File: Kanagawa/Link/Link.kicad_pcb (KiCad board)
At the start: 2 copper layers, 23 x 24 mm, 2 parts, among them J0 Conn_02x10_Counter_Clockwise, J1 Conn_02x10_Counter_Clockwise

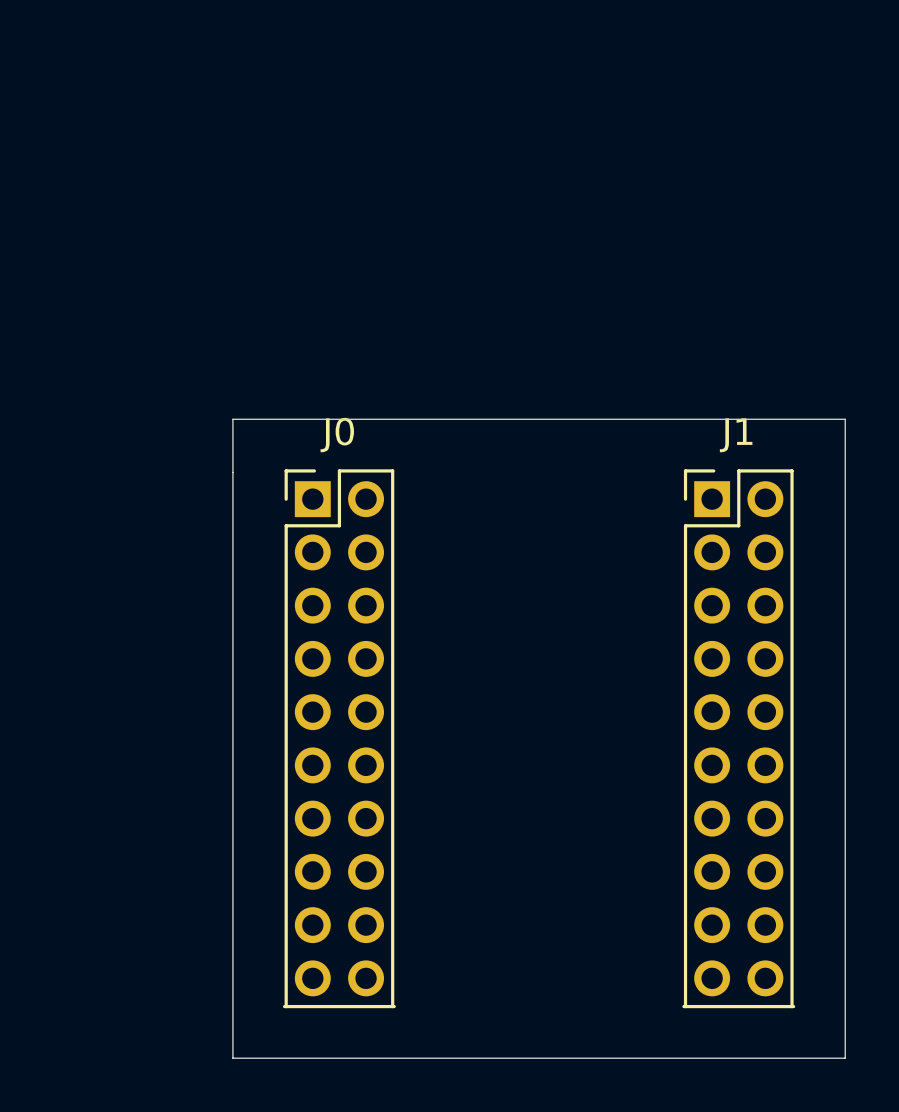
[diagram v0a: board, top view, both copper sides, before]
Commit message: link bridge
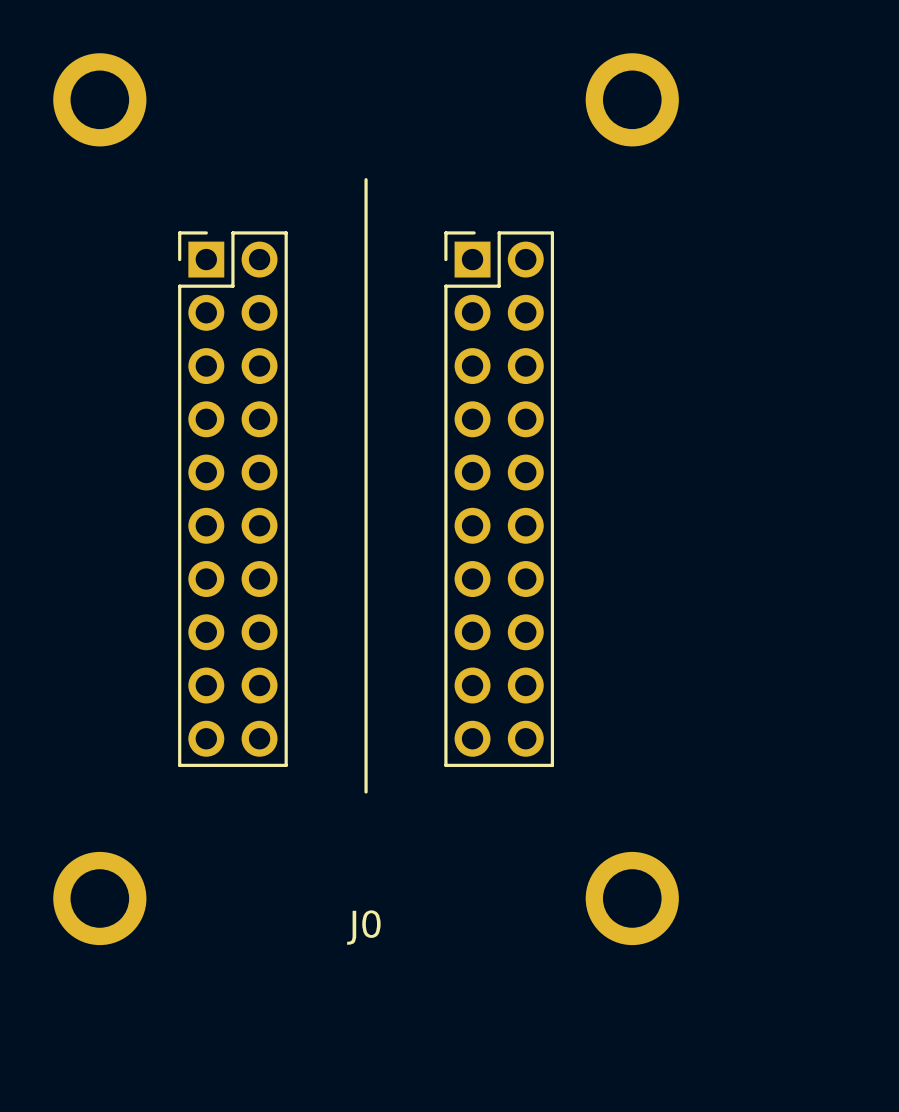
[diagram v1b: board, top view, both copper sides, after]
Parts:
- removed J1: Conn_02x10_Counter_Clockwise, link:conn_2x10_P2.00mm_Vertical
- J0: footprint link:conn_2x10_P2.00mm_Vertical -> link:bridge_2x10_P2.00mm
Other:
- board outline removed
